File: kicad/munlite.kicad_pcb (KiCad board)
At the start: 2 copper layers, 45.7 x 24.9 mm, 21 parts, among them J1 Conn_Pover, J2 Conn_Pir, J3 Conn_Prog, J4 Conn_Opto, J5 Conn_Led, SW1 SW_Push, U1 STM32L031F6Px, U2 AP2112K-3.3, U3 CN5711

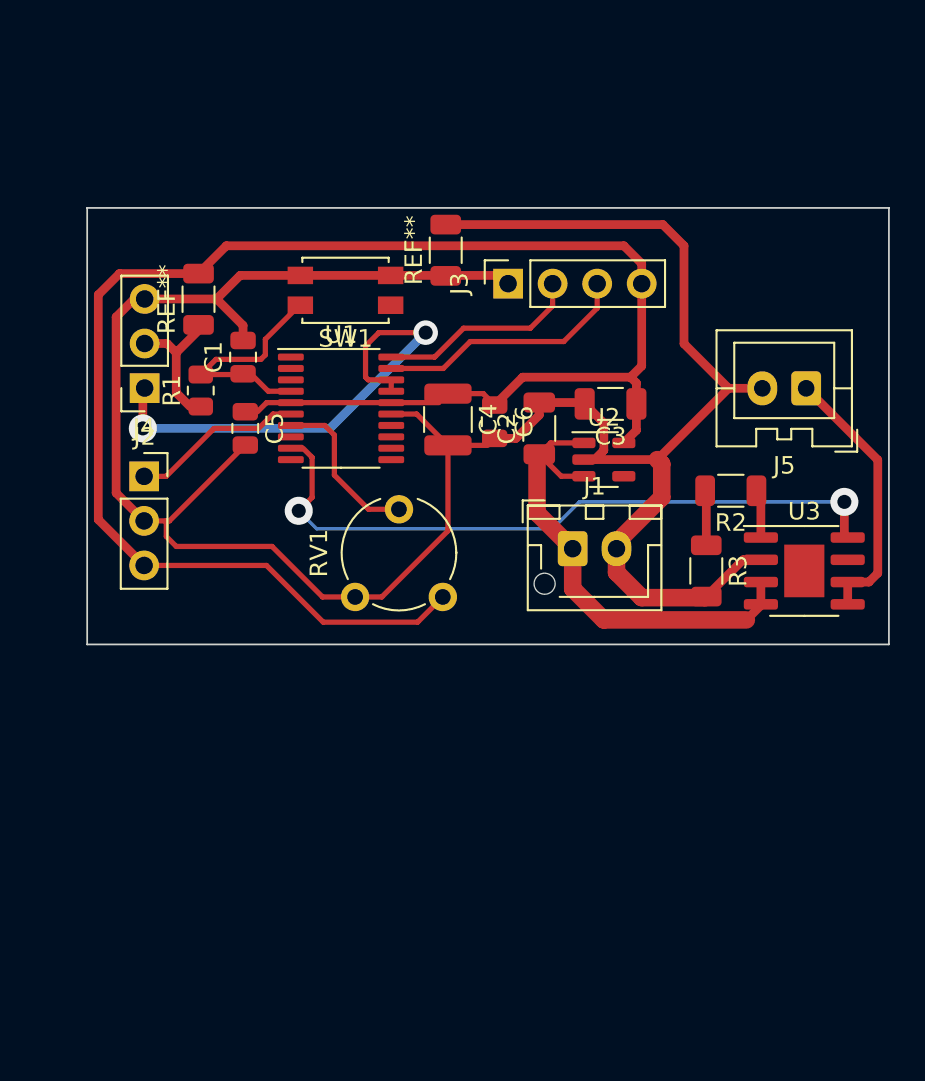
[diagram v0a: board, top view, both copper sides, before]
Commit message: kicad: update pcb
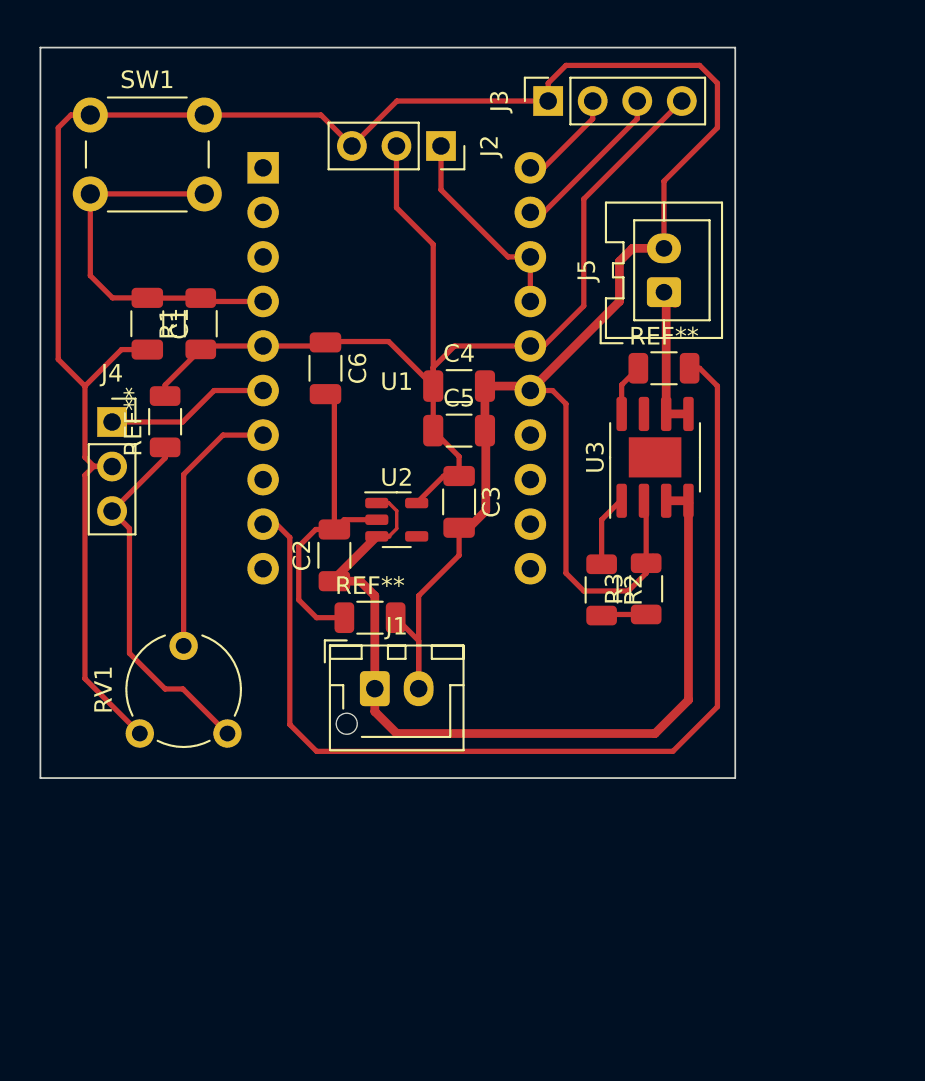
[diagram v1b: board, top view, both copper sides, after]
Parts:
- removed the REF** at (60.2, 35.4)
- removed the REF** at (46.1, 38.2)
- added REF**: R_1206_3216Metric, Resistor_SMD:R_1206_3216Metric, F.Cu at (72.6, 42.2)
- added REF**: R_1206_3216Metric, Resistor_SMD:R_1206_3216Metric, F.Cu at (55.9, 56.4)
- added REF**: R_1206_3216Metric, Resistor_SMD:R_1206_3216Metric, F.Cu at (44.2, 45.2)
- C1, C5, C6: footprint Capacitor_SMD:C_0805_2012Metric -> Capacitor_SMD:C_1206_3216Metric
- C4: footprint Capacitor_SMD:C_1210_3225Metric -> Capacitor_SMD:C_1206_3216Metric
- R1: footprint Resistor_SMD:R_0805_2012Metric -> Resistor_SMD:R_1206_3216Metric
- SW1: footprint Button_Switch_SMD:SW_SPST_EVQP2 -> Button_Switch_THT:SW_PUSH_6mm
- U1: footprint Package_SO:TSSOP-20_4.4x6.5mm_P0.65mm -> Connector_PinHeader_2.54mm:tssop20_adapter
- moved J2 21.8 mm to (59.9, 29.5), turned to -90 degrees
- moved SW1 17.7 mm to (39.9, 27.7), turned to 0 degrees
- moved RV1 14.5 mm to (47.8, 63.0)
- moved J1 13.8 mm to (56.2, 60.4)
- moved C2 13.7 mm to (53.8, 52.8)
- moved U2 12.3 mm to (57.4, 50.8)
- moved C5 12.2 mm to (61.0, 45.7), turned to 0 degrees
- moved U3 10.7 mm to (72.1, 47.2), turned to 90 degrees
- moved J3 10.7 mm to (66.0, 26.9)
- moved C3 10.3 mm to (61.0, 49.8), turned to -90 degrees
- moved C6 10.1 mm to (53.3, 42.2)
- moved J5 9.79 mm to (72.6, 37.8), turned to 90 degrees
- moved R2 9.29 mm to (69.1, 54.8), turned to -90 degrees
- moved C1 5.78 mm to (43.2, 39.6), turned to -90 degrees
- moved R1 3.81 mm to (46.2, 39.6)
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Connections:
- C1 pad 1: GND -> Net-(C1-Pad1)
- R1 pad 2: GND -> Net-(C1-Pad1)
- SW1 pad 2: GND -> Net-(C1-Pad1)
- U1 pad 4: GND -> Net-(C1-Pad1)
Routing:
- net +3V3: track 110.9 -> 87.3 mm
- net Led: track 39.1 -> 61.9 mm, vias 2 -> 0
- net Net-(C1-Pad1): track 0.00 -> 21.6 mm
- net GND: track 154.7 -> 176.2 mm
- net +4V: track 27.6 -> 48.9 mm
- net Pir: track 28.4 -> 11.7 mm, vias 2 -> 0
- net Net-(J5-Pad1): track 15.4 -> 9.16 mm
- net Sens: track 9.48 -> 15.2 mm
- net SWCLK: track 11.7 -> 6.24 mm
- net SWDIO: track 14.6 -> 9.83 mm
- net Net-(R2-Pad1): track 2.77 -> 4.13 mm
- net Net-(R2-Pad2): track 3.14 -> 2.57 mm
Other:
- board size 45.7 x 24.9 mm -> 39.6 x 41.7 mm

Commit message: update pcb
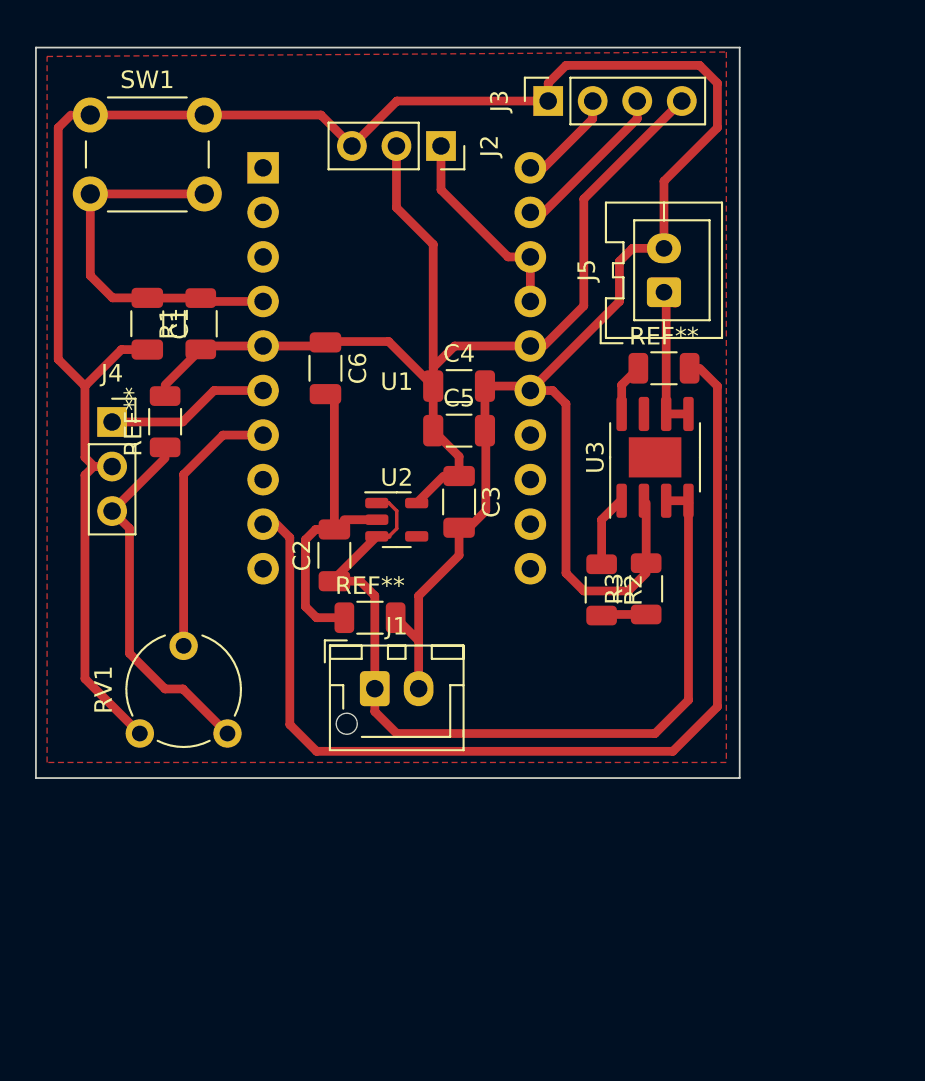
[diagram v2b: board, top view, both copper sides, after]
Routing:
- added copper zone on F.Cu, net GND
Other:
- board size 39.6 x 41.7 mm -> 40.1 x 41.7 mm

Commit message: update board
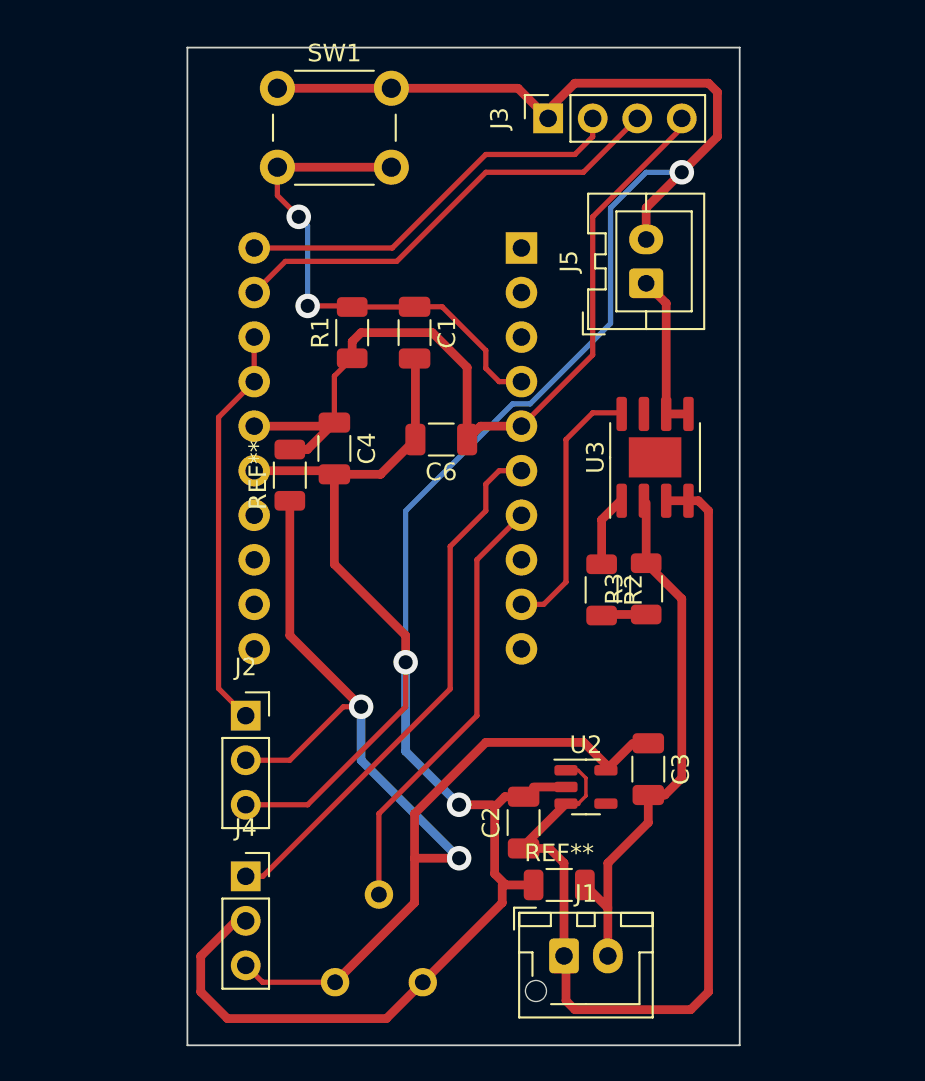
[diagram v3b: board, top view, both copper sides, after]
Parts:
- removed C5: 0.1uF, Capacitor_SMD:C_1206_3216Metric
- removed the REF** at (72.6, 42.2)
- removed the REF** at (44.2, 45.2)
- added REF**: R_1206_3216Metric, Resistor_SMD:R_1206_3216Metric, F.Cu at (51.3, 48.3)
- RV1, U1: moved to B.Cu
- moved J2 34.3 mm to (48.8, 62.0), turned to 0 degrees
- moved J4 27.0 mm to (48.8, 71.1)
- moved C2 18.7 mm to (64.6, 68.1)
- moved U2 18.7 mm to (68.2, 66.0)
- moved C3 18.7 mm to (71.7, 65.0)
- moved REF** 18.7 mm to (66.7, 71.6)
- moved J1 18.7 mm to (66.9, 75.7)
- moved RV1 15.5 mm to (53.9, 77.2)
- moved C1 15.2 mm to (58.4, 40.1)
- moved SW1 10.8 mm to (50.6, 26.2)
- moved R1 8.65 mm to (54.9, 40.1)
- moved C4 7.95 mm to (53.8, 46.7), turned to -90 degrees
- moved C6 7.75 mm to (59.9, 46.2), turned to 180 degrees
- moved U1 4.60 mm to (56.9, 48.0), turned to 180 degrees
- moved J5 1.14 mm to (71.6, 37.3)
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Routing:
- net Led: track 61.9 -> 15.0 mm
- net +3V3: track 87.3 -> 117.6 mm, vias 0 -> 2
- net GND: track 175.9 -> 198.4 mm, vias 0 -> 3
- net Opto: track 9.35 -> 31.0 mm
- net SWCLK: track 6.24 -> 23.0 mm
- net SWDIO: track 9.83 -> 26.0 mm
- net Pir: track 11.7 -> 23.1 mm
- net Sens: track 15.2 -> 25.0 mm
- net +4V: track 48.9 -> 57.2 mm
- net Net-(C1-Pad1): track 21.6 -> 29.7 mm, vias 0 -> 2
- removed copper zone on F.Cu, net GND
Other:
- board size 40.1 x 41.7 mm -> 31.5 x 56.9 mm
